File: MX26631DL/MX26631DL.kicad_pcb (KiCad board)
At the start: 4 copper layers, 21 x 22.6 mm, 14 parts, among them U2 MX26631DL, U4 TPESD0402G15V

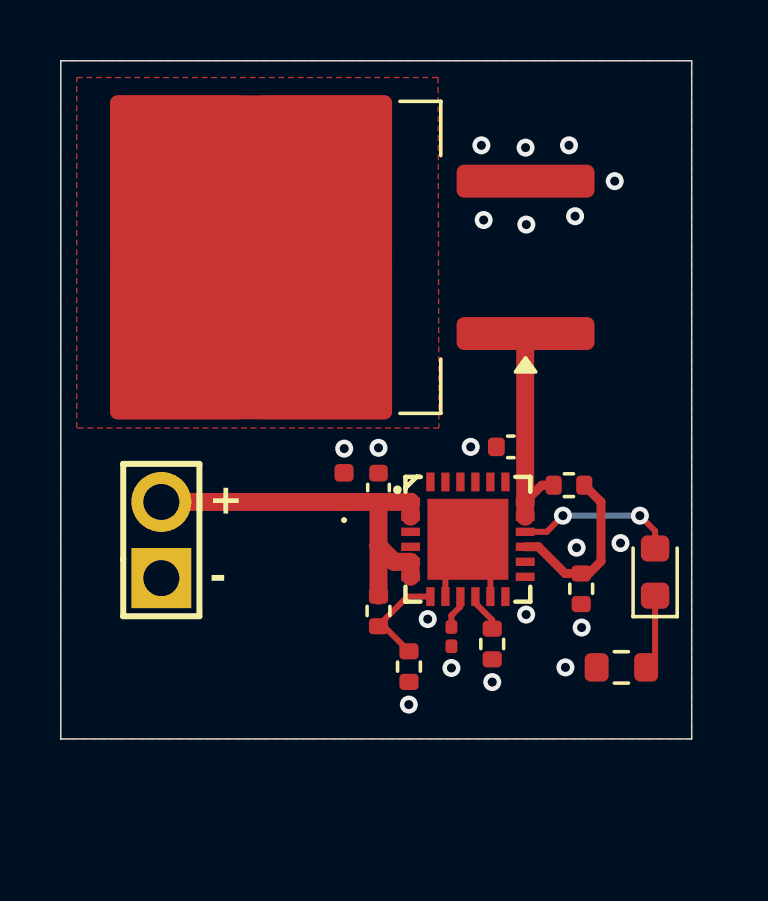
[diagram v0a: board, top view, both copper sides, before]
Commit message: Need to verify circuit 1 more time
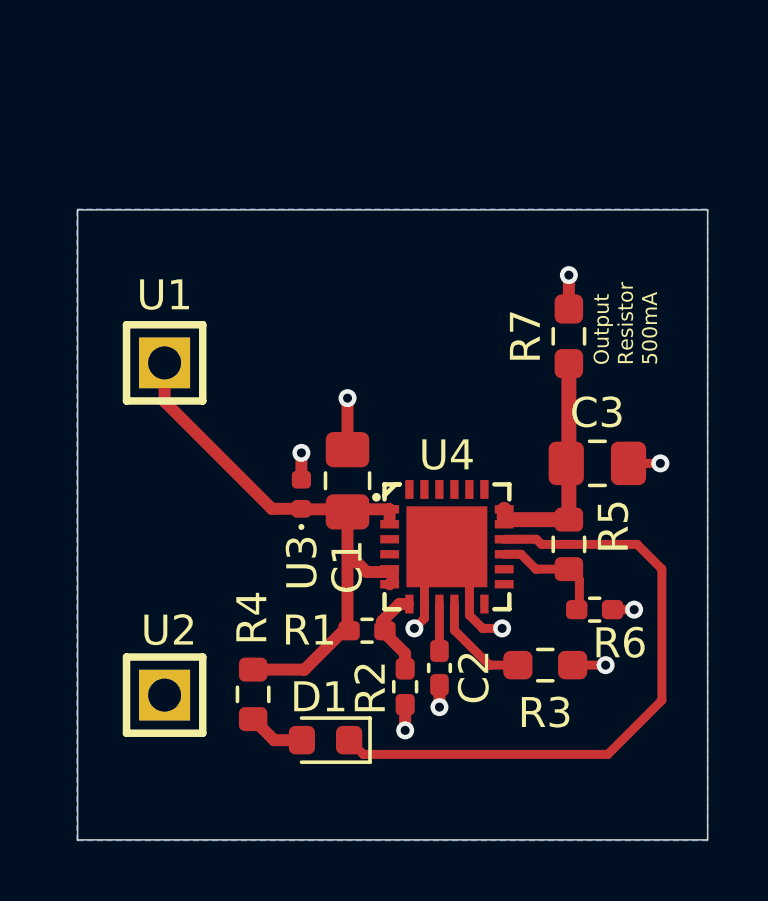
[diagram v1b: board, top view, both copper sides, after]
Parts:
- removed C15, C16: 10uF, Capacitor_SMD:C_0402_1005Metric
- removed H1: X6511WV-02H-C30D60, easyeda2kicad:HDR-TH_2P-P2.54-V-M
- removed R10: 6.2kR, Resistor_SMD:R_0402_1005Metric
- removed R11: 27kR, Resistor_SMD:R_0402_1005Metric
- removed R12, R14: 10kR, Resistor_SMD:R_0402_1005Metric
- removed R13: 39kR, Resistor_SMD:R_0402_1005Metric
- added C2: 100nF, Capacitor_SMD:C_0402_1005Metric_Pad0.74x0.62mm_HandSolder, F.Cu at (107.1, 98.3)
- added C3: 10uF, Capacitor_SMD:C_0805_2012Metric_Pad1.18x1.45mm_HandSolder, F.Cu at (112.3, 91.5)
- added R3: 20kR, Resistor_SMD:R_0603_1608Metric_Pad0.98x0.95mm_HandSolder, F.Cu at (110.6, 98.2)
- added R4: 2kR, Resistor_SMD:R_0603_1608Metric, F.Cu at (100.8, 99.2)
- added R5: 31.6kR, Resistor_SMD:R_0603_1608Metric, F.Cu at (111.4, 94.2)
- added R6: 10kR, Resistor_SMD:R_0402_1005Metric_Pad0.72x0.64mm_HandSolder, F.Cu at (112.2, 96.3)
- added R7: 10R, Resistor_SMD:R_0603_1608Metric_Pad0.98x0.95mm_HandSolder, F.Cu at (111.4, 87.2)
- added U1: ZX-PZ2.54-1-1PZZ, easyeda2kicad:HDR-TH_1P-P2.54-V-M, F.Cu at (97.9, 88.1)
- added U3: TPESD0402G15V, Diode_SMD:D_0402_1005Metric, F.Cu at (102.5, 92.5)
- C1: value 100nF -> 10uF; footprint Capacitor_SMD:C_0201_0603Metric -> Capacitor_SMD:C_0805_2012Metric_Pad1.18x1.45mm_HandSolder
- R1: value 2kR -> 39kR; footprint Resistor_SMD:R_0603_1608Metric -> Resistor_SMD:R_0402_1005Metric_Pad0.72x0.64mm_HandSolder
- R2: value 2R -> 10kR; footprint Package_TO_SOT_SMD:TO-263-2 -> Resistor_SMD:R_0402_1005Metric_Pad0.72x0.64mm_HandSolder
- U2: value MX26631DL -> ZX-PZ2.54-1-1PZZ; footprint easyeda2kicad:QFN-24_L4.0-W4.0-P0.50-TL-EP2.7 -> easyeda2kicad:HDR-TH_1P-P2.54-V-M
- U4: value TPESD0402G15V -> MX26631DL; footprint Diode_SMD:D_0402_1005Metric -> easyeda2kicad:QFN-24_L4.0-W4.0-P0.50-TL-EP2.7
- moved R2 14.8 mm to (105.9, 98.9), turned to -90 degrees
- moved D1 12.3 mm to (103.3, 100.7), turned to 180 degrees
- moved U2 11.4 mm to (97.9, 99.2)
- moved R1 8.57 mm to (104.6, 97.0), turned to 0 degrees
- moved C1 6.24 mm to (104.0, 92.0), turned to 90 degrees
- moved U4 3.96 mm to (107.3, 94.2), turned to 0 degrees
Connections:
- C1 pad 1: Net-(U2-dVdT) -> /+5V_unprot
- D1 pad 1: Net-(D1-K) -> /PGOOD
- D1 pad 2: /PGOOD -> Net-(D1-A)
- R1 pad 1: Net-(D1-K) -> /+5V_unprot
- R1 pad 2: GND -> Net-(U4-OVP)
- R2 pad 1: Net-(C16-Pad1) -> Net-(U4-OVP)
- R2 pad 2: Heatsink -> GND
- U2 pad 1: /+5V_unprot -> GND
- U4 pad 2: GND -> /+5V_unprot
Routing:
- net /PGOOD: track 5.35 -> 21.4 mm, vias 2 -> 0
- net GND: track 4.44 -> 15.6 mm, vias 19 -> 10
- net Net-(C3-Pad1): track 0.00 -> 7.66 mm
- net Net-(C16-Pad1): track 7.29 -> 0.00 mm
- net /+5V_unprot: track 13.7 -> 20.7 mm
- net Net-(U2-PGTH): track 5.83 -> 0.00 mm
- net Net-(U4-PGTH): track 0.00 -> 3.86 mm
- net Net-(U2-OVP): track 3.55 -> 0.00 mm
- net Net-(U4-ILIM): track 0.00 -> 3.47 mm
- net Net-(U4-OVP): track 0.00 -> 2.99 mm
- net Net-(D1-K): track 2.51 -> 0.00 mm
- net Net-(D1-A): track 0.00 -> 1.91 mm
- net Net-(U4-dVdT): track 0.00 -> 1.65 mm
- net Net-(U2-ILIM): track 1.31 -> 0.00 mm
- net Net-(U2-dVdT): track 1.14 -> 0.00 mm
- added copper zone on B.Cu, net GND
- removed copper zone on F.Cu, net GND
- removed copper zone on In1.Cu, net GND
- removed copper zone on In2.Cu, net GND
- removed copper zone on F.Cu, net Heatsink
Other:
- board size 21 x 22.6 mm -> 21 x 21 mm
- copper layers 4 -> 2
- board text added: "Output Resistor 500mA"
- board text removed: "+"
- board text removed: "-"
